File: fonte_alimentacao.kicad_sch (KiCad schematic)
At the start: 1 part, among them J1 Conn_01x03

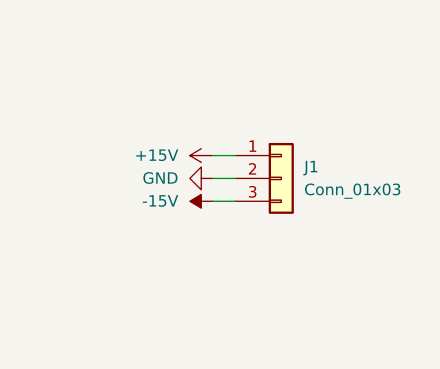
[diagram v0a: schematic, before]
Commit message: Definicao subbass e filtro passa baixo
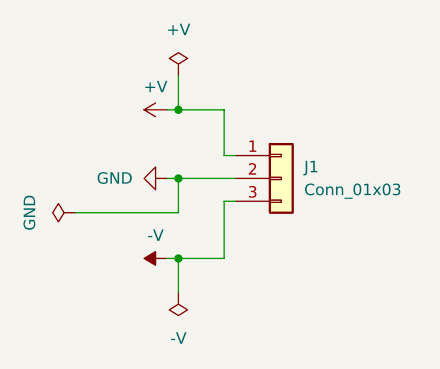
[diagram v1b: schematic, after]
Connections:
- net +15V renamed +V
- net -15V renamed -V
